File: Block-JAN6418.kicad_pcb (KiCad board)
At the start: 2 copper layers, 50 x 65 mm, 21 parts, among them U1 JAN6418, U2 LM317L

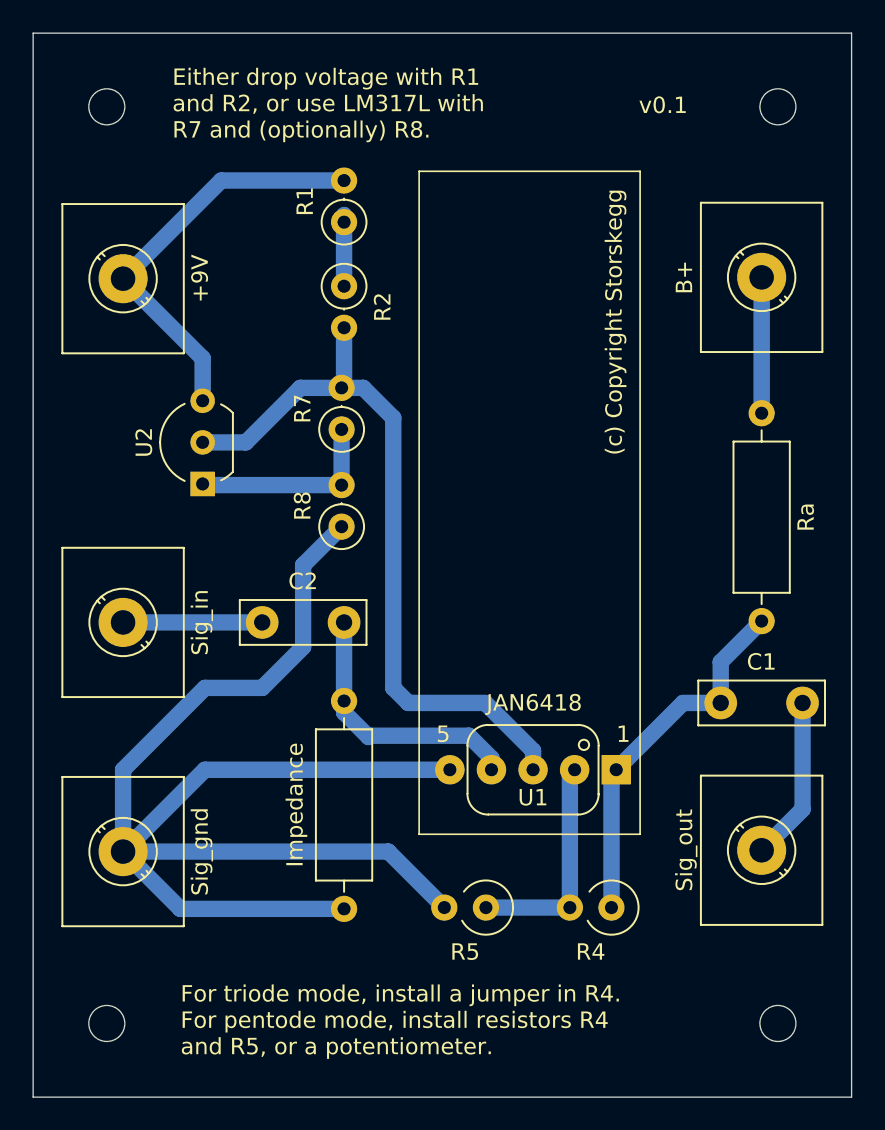
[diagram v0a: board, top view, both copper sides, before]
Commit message: shrinkage
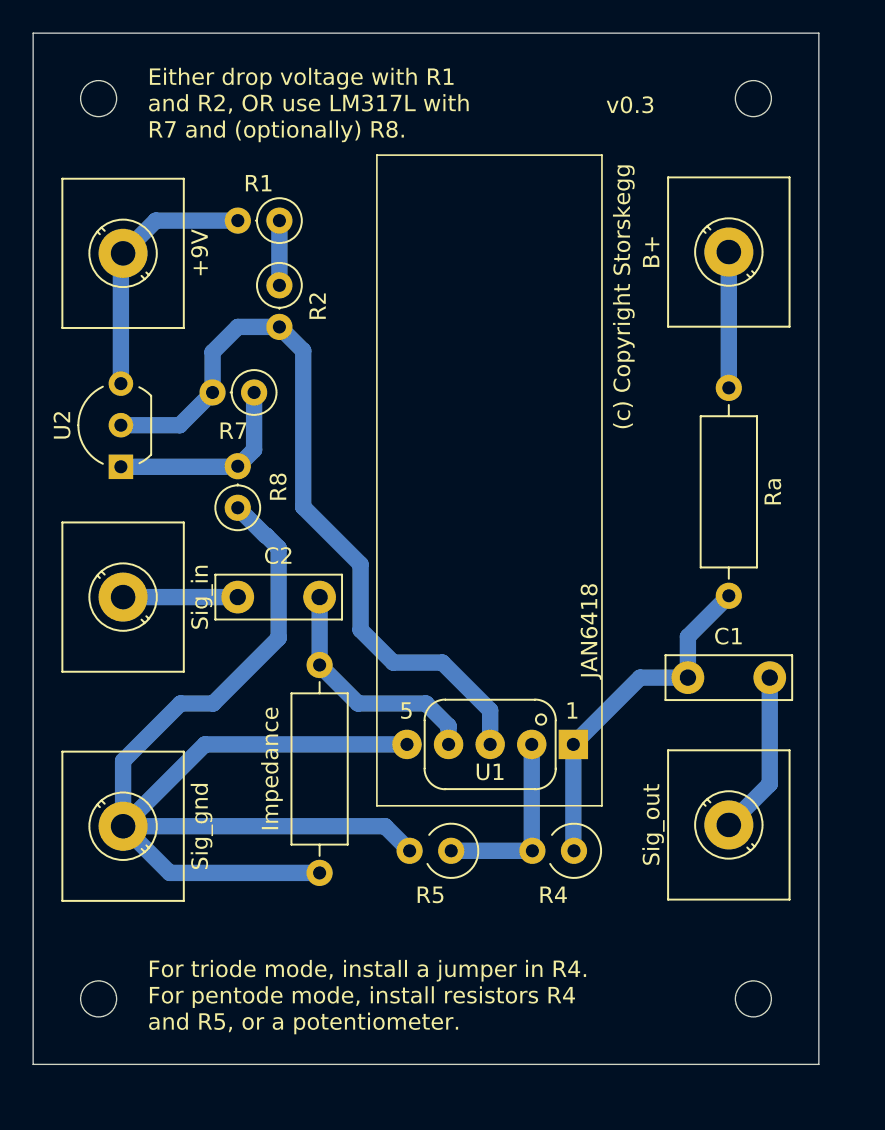
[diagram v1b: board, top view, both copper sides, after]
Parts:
- moved R8 6.45 mm to (62.5, 64.0)
- moved R7 5.80 mm to (63.5, 57.0), turned to 180 degrees
- moved U2 5.10 mm to (55.4, 61.5)
- moved R4 4.16 mm to (83.0, 85.0)
- moved R5 4.06 mm to (75.5, 85.0)
- moved R1 3.95 mm to (65.0, 46.5), turned to 180 degrees
- moved R2 3.95 mm to (65.0, 50.4)
- moved U1 3.04 mm to (83.0, 78.5)
- moved Impedance 2.66 mm to (67.5, 73.6)
- moved B+ 2.53 mm to (92.5, 48.4)
- moved C1 2.53 mm to (90.0, 74.4)
- moved Ra 2.53 mm to (92.5, 56.7)
- moved Sig_out 2.53 mm to (92.5, 83.4)
- moved C2 2.15 mm to (62.5, 69.5)
- moved REF** 2.12 mm to (94.0, 94.0)
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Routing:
- net +9V: track 25.5 -> 15.7 mm
- net GND: track 85.5 -> 76.4 mm
- net Net-(U1A-G2): track 13.7 -> 11.4 mm
- net Net-(U1A-G1): track 16.2 -> 14.7 mm
- net Net-(J3-Pin_1): track 8.50 -> 7.01 mm
- net Net-(U1A-P): track 22.7 -> 21.2 mm
- net Net-(U2-VO): track 45.3 -> 46.2 mm
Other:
- board size 50 x 65 mm -> 48 x 63 mm
- board text added: "Either drop voltage with R1 and R2, OR use LM317L with R7 and (optionally) R8."
- board text added: "v0.3"
- board text removed: "Either drop voltage with R1 and R2, or use LM317L with R7 and (optionally) R8."
- board text removed: "v0.1"
